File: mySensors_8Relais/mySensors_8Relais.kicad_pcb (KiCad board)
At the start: 2 copper layers, 81.3 x 59.7 mm, 16 parts

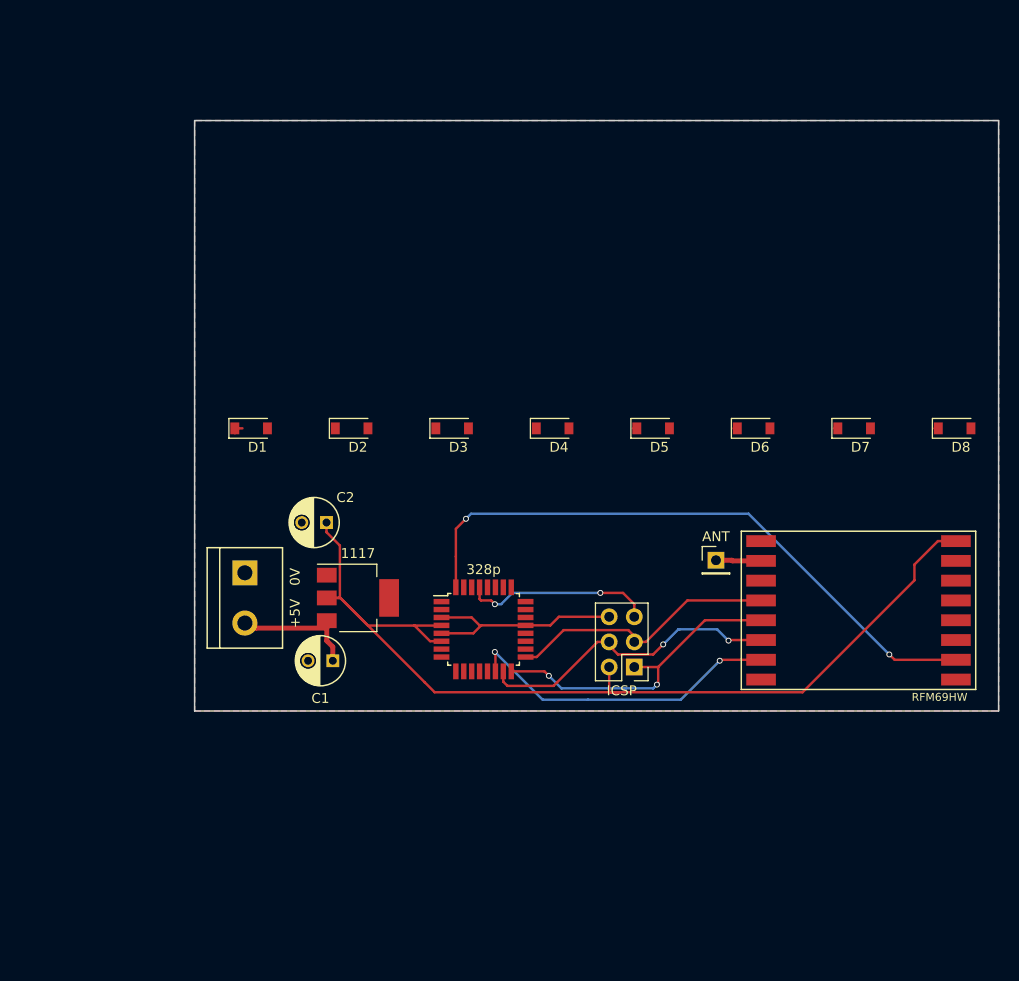
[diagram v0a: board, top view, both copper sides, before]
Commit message: Terminé le circuit 8 Relais
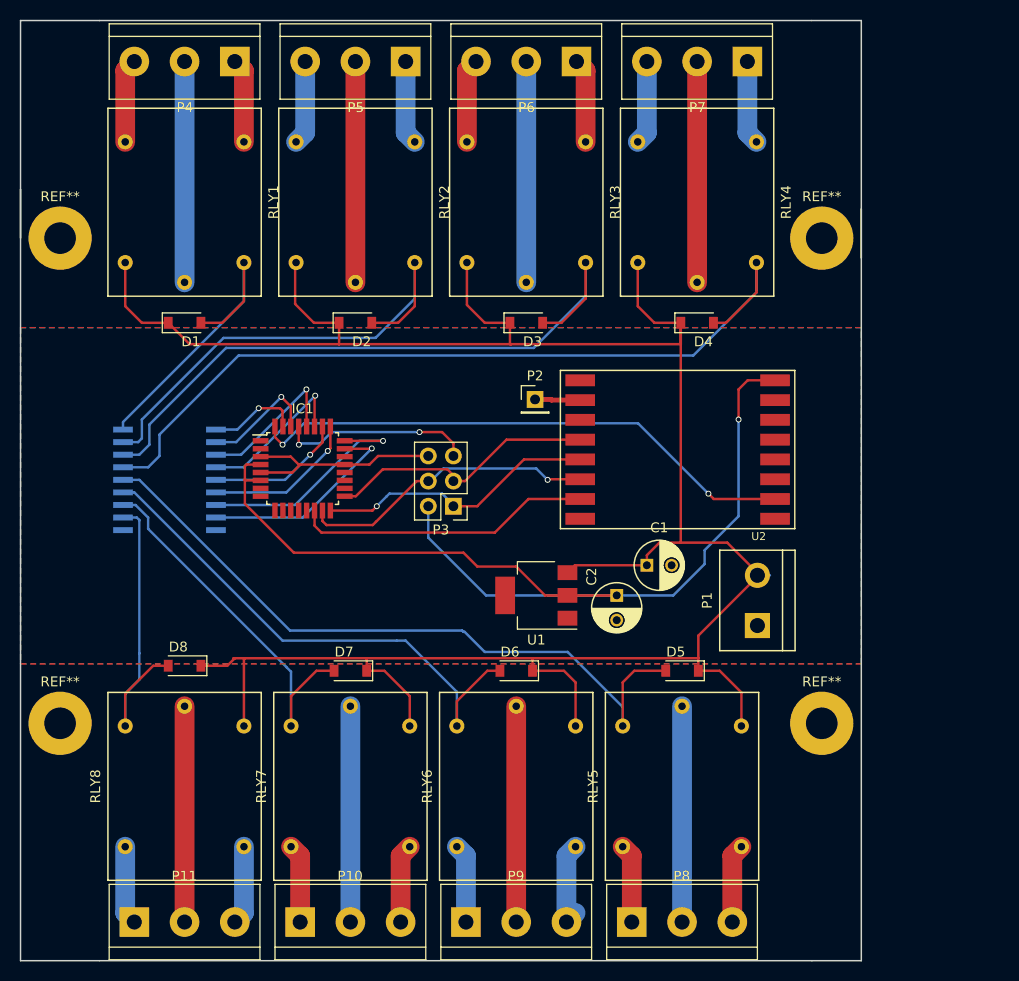
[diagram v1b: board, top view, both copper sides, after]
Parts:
- added IC2: ULN2803A, Housings_SOIC:SOIC-18W_7.5x11.6mm_Pitch1.27mm, B.Cu at (135.9, 102.4)
- added P10: CONN_01X03, Connectors:bornier3, F.Cu at (149.1, 147.1)
- added P11: CONN_01X03, Connectors:bornier3, F.Cu at (132.3, 147.1)
- added P4: CONN_01X03, Connectors:bornier3, F.Cu at (142.5, 60.1)
- added P5: CONN_01X03, Connectors:bornier3, F.Cu at (159.8, 60.1)
- added P6: CONN_01X03, Connectors:bornier3, F.Cu at (177.0, 60.1)
- added P7: CONN_01X03, Connectors:bornier3, F.Cu at (194.3, 60.1)
- added P8: CONN_01X03, Connectors:bornier3, F.Cu at (182.6, 147.1)
- added P9: CONN_01X03, Connectors:bornier3, F.Cu at (165.9, 147.1)
- added REF**: MountingHole_3.2mm_M3_Pad, Mounting_Holes:MountingHole_3.2mm_M3_Pad, F.Cu at (201.8, 77.9)
- added REF**: MountingHole_3.2mm_M3_Pad, Mounting_Holes:MountingHole_3.2mm_M3_Pad, F.Cu at (124.8, 77.9)
- added REF**: MountingHole_3.2mm_M3_Pad, Mounting_Holes:MountingHole_3.2mm_M3_Pad, F.Cu at (124.8, 127.0)
- added REF**: MountingHole_3.2mm_M3_Pad, Mounting_Holes:MountingHole_3.2mm_M3_Pad, F.Cu at (201.8, 127.0)
- added RLY1: SRD_Type_C, MyLibrary:SRD_Relay_TypeC, F.Cu at (137.4, 74.3)
- added RLY2: SRD_Type_C, MyLibrary:SRD_Relay_TypeC, F.Cu at (154.7, 74.3)
- added RLY3: SRD_Type_C, MyLibrary:SRD_Relay_TypeC, F.Cu at (172.0, 74.3)
- added RLY4: SRD_Type_C, MyLibrary:SRD_Relay_TypeC, F.Cu at (189.2, 74.3)
- added RLY5: SRD_Type_C, MyLibrary:SRD_Relay_TypeC, F.Cu at (187.7, 133.3)
- added RLY6: SRD_Type_C, MyLibrary:SRD_Relay_TypeC, F.Cu at (170.9, 133.3)
- added RLY7: SRD_Type_C, MyLibrary:SRD_Relay_TypeC, F.Cu at (154.2, 133.3)
- added RLY8: SRD_Type_C, MyLibrary:SRD_Relay_TypeC, F.Cu at (137.4, 133.3)
- P1: renamed from +5V   0V
- moved D8 81.5 mm to (137.4, 121.2), turned to 180 degrees
- moved D7 56.5 mm to (154.2, 121.7), turned to 180 degrees
- moved P1 51.8 mm to (195.3, 114.6), turned to 90 degrees
- moved D6 34.3 mm to (170.9, 121.7), turned to 180 degrees
- moved C1 33.2 mm to (184.2, 111.0), turned to 0 degrees
- moved C2 30.2 mm to (181.1, 114.0), turned to 270 degrees
- moved D5 24.7 mm to (187.7, 121.7), turned to 180 degrees
- moved U2 24.5 mm to (195.7, 106.3)
- moved IC1 24.5 mm to (149.4, 101.2)
- moved P2 24.5 mm to (172.8, 94.2)
- moved P3 24.5 mm to (164.6, 105.0)
- moved D4 18.1 mm to (189.2, 86.5)
- moved U1 18.0 mm to (173.0, 114.0), turned to 180 degrees
- moved D3 13.0 mm to (172.0, 86.5)
- moved D1 12.6 mm to (137.4, 86.5)
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- renumbered 328p to IC1, ANT to P2, ICSP to P3, 1117 to U1, RFM69HW to U2
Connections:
- C1 pad 1: VCC -> /VCC
- C1 pad 2: GND -> /GND
- C2 pad 2: GND -> /GND
- D1 pad 1: /S0 -> /VCC
- D1 pad 2: GND -> /S0
- D2 pad 1: /S1 -> /VCC
- D2 pad 2: GND -> /S1
- D3 pad 1: /S2 -> /VCC
- D3 pad 2: GND -> /S2
- D4 pad 1: /S3 -> /VCC
- D4 pad 2: GND -> /S3
- D5 pad 1: /S4 -> /VCC
- D5 pad 2: GND -> /S4
- D6 pad 1: /S5 -> /VCC
- D6 pad 2: GND -> /S5
- D7 pad 1: /S6 -> /VCC
- D7 pad 2: GND -> /S6
- D8 pad 1: /S7 -> /VCC
- D8 pad 2: GND -> /S7
- IC1 pad 21: GND -> /GND
- IC1 pad 23: /SER -> /SL7
- IC1 pad 24: /RCLK -> /SL6
- IC1 pad 25: /SRCLK -> /SL5
- IC1 pad 26: Net-(IC1-Pad26) -> /SL4
- IC1 pad 27: Net-(IC1-Pad27) -> /SL3
- IC1 pad 28: Net-(IC1-Pad28) -> /SL2
- IC1 pad 3: GND -> /GND
- IC1 pad 30: Net-(IC1-Pad30) -> /SL1
- IC1 pad 31: Net-(IC1-Pad31) -> /SL0
- IC1 pad 5: GND -> /GND
- P1 pad 1: GND -> /GND
- P1 pad 2: VCC -> /VCC
- P3 pad 6: GND -> /GND
- U1 pad 1: GND -> /GND
- U1 pad 3: VCC -> /VCC
- U2 pad 11: GND -> /GND
- U2 pad 9: GND -> /GND
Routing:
- net /VCC: track 0.00 -> 241.9 mm
- net /S3: track 0.00 -> 84.3 mm
- net /S4: track 0.39 -> 71.2 mm
- net /S2: track 0.35 -> 67.0 mm
- net /S5: track 0.39 -> 53.7 mm
- net /S1: track 0.00 -> 49.7 mm
- net /S6: track 0.39 -> 38.6 mm
- net /S7: track 0.39 -> 32.0 mm
- net /S0: track 1.28 -> 31.1 mm
- net /SL6: track 0.00 -> 23.5 mm, vias 0 -> 1
- net Net-(P7-Pad2): track 0.00 -> 22.3 mm
- net Net-(P6-Pad2): track 0.00 -> 22.3 mm
- net Net-(P5-Pad2): track 0.00 -> 22.3 mm
- net Net-(P4-Pad2): track 0.00 -> 22.3 mm
- net GND: track 22.0 -> 0.00 mm
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- added copper zone on B.Cu, net /GND
- added copper zone on F.Cu, net /GND
- removed copper zone on B.Cu, net GND
- removed copper zone on F.Cu, net GND
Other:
- board size 81.3 x 59.7 mm -> 85 x 95 mm
